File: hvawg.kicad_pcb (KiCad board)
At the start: 2 copper layers, 150 x 40 mm, 90 parts, among them J1 Conn_01x04_Pin, J10 Conn_01x01_Pin, J2 Conn_01x04_Pin, J3 Conn_01x04_Pin, J4 Conn_01x04_Pin, J5 Conn_01x04_Pin, J6 Conn_01x04_Pin, J7 Conn_01x04_Pin, J8 Conn_01x04_Pin, J9 Conn_01x08_Pin, Q1 IRF730, Q3 IRF9610, U1 L7805, U2 74HC595D,110, U3 DAC0808LCMX/NOPB, U4 NE5532, U6 LM8261, U7 LM8261, U8 NE5532

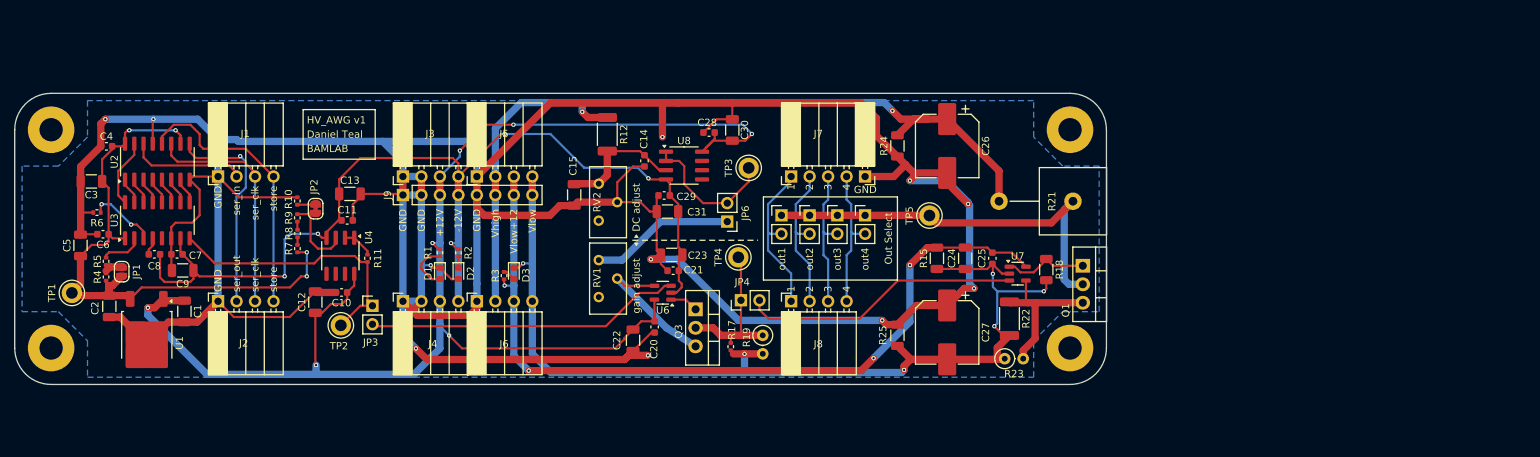
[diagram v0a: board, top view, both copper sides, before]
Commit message: new board
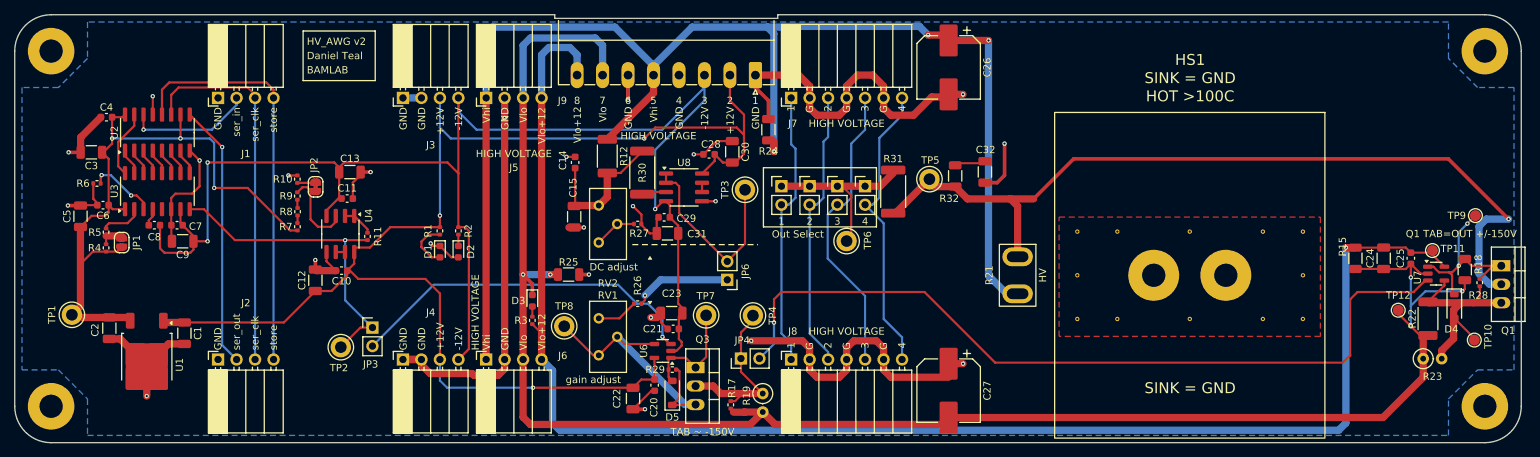
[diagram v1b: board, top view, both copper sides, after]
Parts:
- removed J10: Conn_01x01_Pin, Connector_PinSocket_2.54mm:PinSocket_1x01_P2.54mm_Horizontal
- added C32: DNP, Capacitor_SMD:C_1206_3216Metric, F.Cu at (209.3, 89.8)
- added D4: BZT52C12, Diode_SMD:D_SOD-123, F.Cu at (273.8, 108.2)
- added D5: BZT52C12, Diode_SMD:D_SOD-123, F.Cu at (166.3, 120.2)
- added HS1: Wakefield 272-AB, Library:Heatsink_Wakefield_272-AB, F.Cu at (232.5, 104.0)
- added R26: 3.3k, Resistor_SMD:R_0402_1005Metric, F.Cu at (161.6, 107.9)
- added R27: 820, Resistor_SMD:R_0402_1005Metric, F.Cu at (161.6, 97.0)
- added R28: 100k, Resistor_SMD:R_0402_1005Metric, F.Cu at (277.3, 105.0)
- added R29: 1M, Resistor_SMD:R_0402_1005Metric, F.Cu at (166.3, 117.0)
- added R30: 22k, Resistor_SMD:R_2512_6332Metric, F.Cu at (162.2, 89.9)
- added R31: 4.7k, Resistor_SMD:R_2512_6332Metric, F.Cu at (196.7, 92.5)
- added R32: DNP, Resistor_SMD:R_1206_3216Metric, F.Cu at (205.2, 90.3)
- added TP10: TestPoint, TestPoint:TestPoint_Pad_D1.5mm, F.Cu at (276.6, 112.9)
- added TP11: TestPoint, TestPoint:TestPoint_Pad_D1.5mm, F.Cu at (270.8, 100.6)
- added TP12: TestPoint, TestPoint:TestPoint_Pad_D1.5mm, F.Cu at (266.1, 108.8)
- added TP6: TestPoint, TestPoint:TestPoint_Keystone_5005-5009_Compact, F.Cu at (190.3, 99.3)
- added TP7: TestPoint, TestPoint:TestPoint_Keystone_5005-5009_Compact, F.Cu at (171.0, 109.5)
- added TP8: TestPoint, TestPoint:TestPoint_Keystone_5005-5009_Compact, F.Cu at (151.5, 111.0)
- added TP9: TestPoint, TestPoint:TestPoint_Pad_D1.5mm, F.Cu at (276.7, 95.8)
- J7: value Conn_01x04_Pin -> Conn_01x07_Pin; footprint Library:PinSocket_1x04_P2.54mm_Horizontal_flipped -> Library:PinSocket_1x07_P2.54mm_Horizontal_flipped
- J8: value Conn_01x04_Pin -> Conn_01x07_Pin; footprint Connector_PinSocket_2.54mm:PinSocket_1x04_P2.54mm_Horizontal -> Connector_PinSocket_2.54mm:PinSocket_1x07_P2.54mm_Horizontal
- J9: footprint Connector_PinHeader_2.54mm:PinHeader_1x08_P2.54mm_Vertical -> Library:PhoenixContact_MC_1,5_8-G-3.5_1x08_P3.50mm_Horizontal_EdgeNotch
- Q1, Q3: footprint Package_TO_SOT_THT:TO-220-3_Vertical -> Library:TO-220-3_Vertical_HV
- R21: footprint Resistor_THT:R_Axial_Power_L25.0mm_W9.0mm_P10.16mm_Vertical -> Library:TO-220-2_Horizontal_LTO50
- RV1: value 3k -> 1k
- moved H3 58.0 mm to (278.0, 73.2)
- moved H4 57.6 mm to (278.0, 122.0)
- moved C24 57.5 mm to (264.1, 101.7)
- moved C25 57.5 mm to (267.8, 101.7)
- moved Q1 57.5 mm to (280.3, 102.7)
- moved R15 57.5 mm to (260.2, 101.7)
- moved U7 57.5 mm to (271.3, 103.8)
- moved R18 57.5 mm to (275.2, 103.2)
- moved R22 57.5 mm to (270.2, 110.0)
- moved R23 57.5 mm to (269.5, 115.5)
- moved J9 51.2 mm to (177.8, 76.5), turned to 180 degrees
- moved R25 45.9 mm to (152.1, 103.9), turned to 180 degrees
- moved R24 17.9 mm to (179.6, 84.0), turned to 90 degrees
- moved J7 13.2 mm to (197.9, 79.6)
- moved J5 10.9 mm to (148.4, 79.6)
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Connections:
- C14 pad 1: Net-(U8A-+) -> Net-(C14-Pad1)
- C15 pad 1: Net-(U8A-+) -> Net-(C14-Pad1)
- J5 pad 1: GND -> +100V
- J5 pad 2: +100V -> GND
- J5 pad 3: -100+12V -> -100V
- J5 pad 4: -100V -> -100+12V
- J6 pad 1: GND -> +100V
- J6 pad 2: +100V -> GND
- J6 pad 3: -100+12V -> -100V
- J6 pad 4: -100V -> -100+12V
- J7 pad 2: Net-(J7-Pin_2) -> GND
- J7 pad 4: Net-(J7-Pin_4) -> GND
- J8 pad 2: Net-(J7-Pin_2) -> GND
- J8 pad 4: Net-(J7-Pin_4) -> GND
- J9 pad 2: GND -> +12V
- J9 pad 3: +12V -> -12V
- J9 pad 4: -12V -> GND
- J9 pad 5: GND -> +100V
- J9 pad 6: +100V -> GND
- J9 pad 7: -100+12V -> -100V
- J9 pad 8: -100V -> -100+12V
- JP10 pad 1: Net-(JP10-A) -> output_post
- JP10 pad 2: Net-(J7-Pin_3) -> Net-(J7-Pin_5)
- JP11 pad 1: Net-(JP10-A) -> output_post
- JP11 pad 2: Net-(J7-Pin_4) -> Net-(J7-Pin_7)
- JP8 pad 1: Net-(JP10-A) -> output_post
- JP9 pad 1: Net-(JP10-A) -> output_post
- JP9 pad 2: Net-(J7-Pin_2) -> Net-(J7-Pin_3)
- Q1 pad 2: Net-(JP10-A) -> Net-(Q1-D)
- Q3 pad 3: Net-(Q3-S) -> Net-(D5-K)
- R12 pad 2: Net-(U8A-+) -> Net-(C14-Pad1)
- R21 pad 1: Net-(JP10-A) -> Net-(Q1-D)
- RV1 pad 1: Net-(JP6-A) -> Net-(R26-Pad2)
- RV1 pad 2: Net-(Q3-S) -> Net-(D5-K)
- RV1 pad 3: unconnected-(RV1-Pad3) -> Net-(D5-K)
- RV2 pad 1: Net-(U8A-+) -> Net-(C14-Pad1)
- RV2 pad 2: GND -> Net-(R27-Pad1)
- RV2 pad 3: unconnected-(RV2-Pad3) -> Net-(R27-Pad1)
- TP5 pad 1: Net-(JP10-A) -> Net-(Q1-D)
- U4 pad 5: (no net) -> GND
- U4 pad 6: (no net) -> Net-(U4B--)
- U4 pad 7: (no net) -> Net-(U4B--)
- U6 pad 4: Net-(Q3-S) -> Net-(D5-K)
- U8 pad 5: (no net) -> GND
- U8 pad 6: (no net) -> Net-(U8B--)
- U8 pad 7: (no net) -> Net-(U8B--)
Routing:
- net GND: track 529.9 -> 257.3 mm, vias 12 -> 23
- net Net-(Q1-D): track 0.00 -> 115.3 mm, vias 0 -> 1
- net -100V: track 138.5 -> 248.5 mm, vias 6 -> 5
- net -100+12V: track 110.7 -> 210.5 mm, vias 4 -> 1
- net Net-(JP4-B): track 38.3 -> 112.1 mm, vias 0 -> 1
- net +100V: track 112.5 -> 185.3 mm, vias 2 -> 3
- net Net-(JP10-A): track 67.3 -> 0.00 mm
- net -12V: track 138.7 -> 192.4 mm, vias 5 -> 3
- net Net-(J7-Pin_5): track 0.00 -> 40.8 mm
- net Net-(J7-Pin_7): track 0.00 -> 40.7 mm
- net Net-(D5-K): track 0.00 -> 39.0 mm
- net output_post: track 0.00 -> 35.9 mm
- net Net-(J7-Pin_2): track 20.7 -> 0.00 mm
- net Net-(Q3-S): track 19.8 -> 0.00 mm
- net Net-(J7-Pin_4): track 19.7 -> 0.00 mm
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- added copper zone on F.Cu, net GND
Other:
- board size 150 x 40 mm -> 207 x 58.8 mm
- board text added: "- INSULATE"
- board text added: "5"
- board text added: "6"
- board text added: "7"
- board text added: "8"
- board text added: "G"
- board text added: "HIGH VOLTAGE"
- board text added: "HOT >100C"
- board text added: "HV_AWG v2"
- board text added: "Q1 TAB = OUTPUT +/-150V"
- board text added: "Q1 TAB=OUT +/-150V"
- board text added: "SINK = GND"
- board text added: "TAB ~ -150V"
- board text added: "Vhi"
- board text added: "Vlo"
- board text added: "Vlo+12"
- board text removed: "HV_AWG v1"
- board text removed: "Vhigh"
- board text removed: "Vlow"
- board text removed: "Vlow+12"
- board text removed: "out1"
- board text removed: "out2"
- board text removed: "out3"
- board text removed: "out4"
